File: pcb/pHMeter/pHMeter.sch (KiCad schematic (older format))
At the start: 75 parts, among them J1 Conn_02x03_Odd_Even, J2 Conn_Coaxial_Power, J3 Conn_Coaxial_Power, J4 Conn_Coaxial_Power, J5 RJ12, J6 RJ12, Q1 BSP75, Q2 BSP75, U1 TLV6004PW, U2 TLV6004PW, X1 MINI-USB-SCHIELD-32005-201

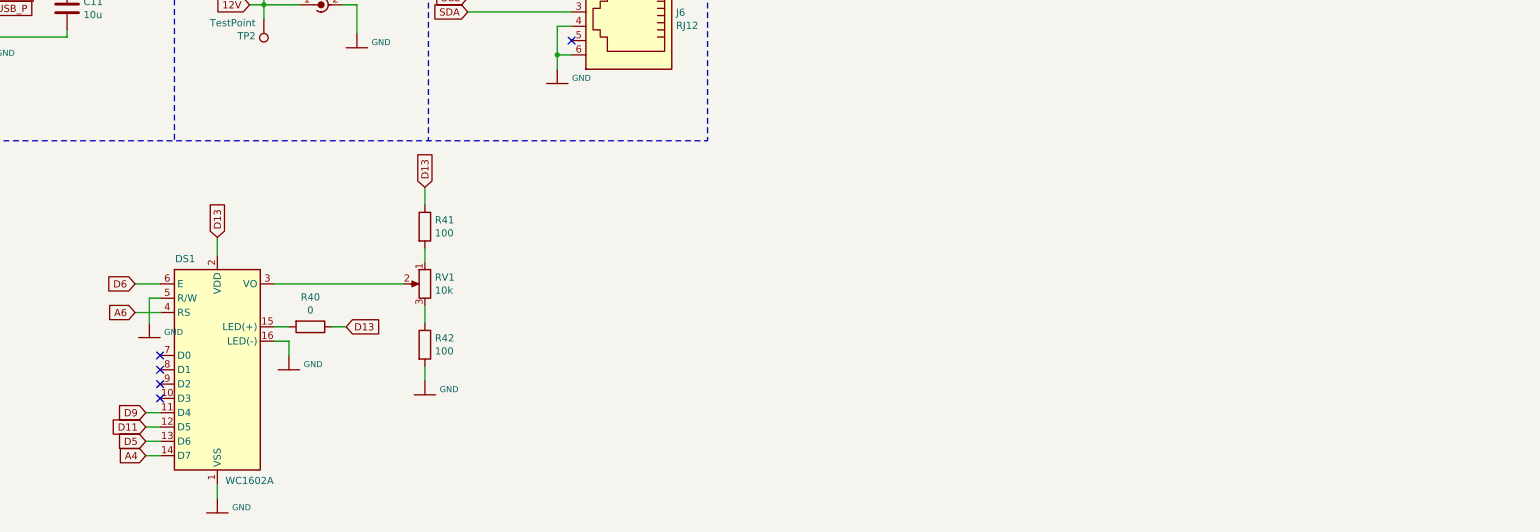
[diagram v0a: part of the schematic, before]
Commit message: change power supply for LCD1602
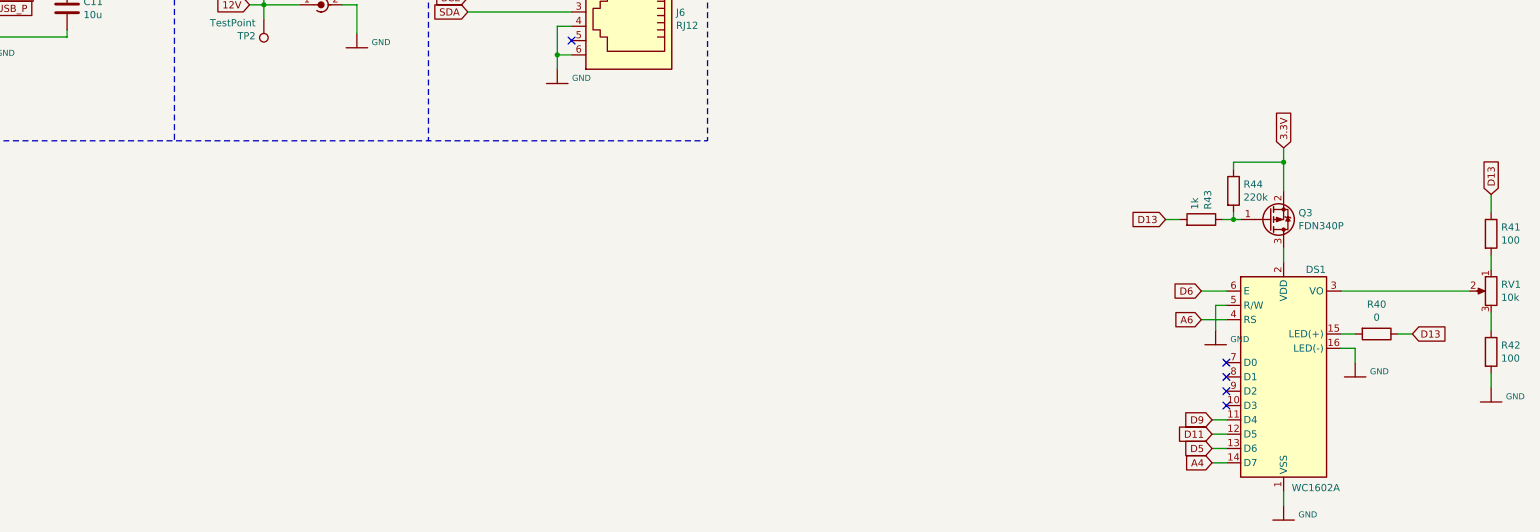
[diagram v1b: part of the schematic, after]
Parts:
- added Q3: FDN340P, Package_TO_SOT_SMD:SOT-23, symbol bioreactor:FDN340P
- added R43: 1k, Resistor_SMD:R_0805_2012Metric_Pad1.15x1.40mm_HandSolder, symbol Device:R
- added R44: 220k, Resistor_SMD:R_0805_2012Metric_Pad1.15x1.40mm_HandSolder, symbol Device:R
- J2, J3: footprint (none) -> Connector_Coaxial:BNC_TEConnectivity_1478204_Vertical
- J4: footprint (none) -> Connector_BarrelJack:BarrelJack_Horizontal
- J5, J6: footprint (none) -> Connector_RJ:RJ12_Amphenol_54601
- JP1, JP2, JP3, JP4: footprint (none) -> Connector_PinHeader_2.54mm:PinHeader_1x02_P2.54mm_Vertical
- LED1, LED2, LED3, LED4, LED5, LED6, LED7: footprint (none) -> LED_SMD:LED_0805_2012Metric_Pad1.15x1.40mm_HandSolder
- R1, R10, R11, R12, R13, R14, R15, R16, R17, R18, R19, R2, R20, R21, R22, R23, R24, R25, R26, R27, R28, R3, R4, R40, R41, R42, R5, R6, R7, R8, R9, RV1: footprint (none) -> Resistor_SMD:R_0805_2012Metric_Pad1.15x1.40mm_HandSolder
- TP1, TP2: footprint (none) -> TestPoint:TestPoint_Pad_D1.5mm
- X1: footprint (none) -> Connector_USB:USB_Mini-B_Lumberg_2486_01_Horizontal
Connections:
- net +3V3: now also Q3.2 (S), R44.1
- net D13: now also R43.2; no longer DS1.2 (VDD)
- new net: DS1.2 (VDD), Q3.3 (D)
- new net: Q3.1 (G), R43.1, R44.2
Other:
- moved on the sheet: DS1, R40, R41, R42, RV1
